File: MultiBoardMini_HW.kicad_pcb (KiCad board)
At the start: 2 copper layers, 63 x 63 mm, 52 parts, among them J1 PB0, J2 PA10, J3 Conn_01x02_Male, J4 PA10, J6 Conn_01x04, SW1 PF1, SW2 RESET, SW3 SW_Push_DPDT, SW5 SW_Push_DPDT, T3 PTS_1.5_2, U1 M78AR5-1, U2 NUCLEO-F303K8, U3 ESP32-C3-WROOM-02-N4, U4 TB67H303HG, U5 TB67H303HG, U6 MCP2562-E_SN

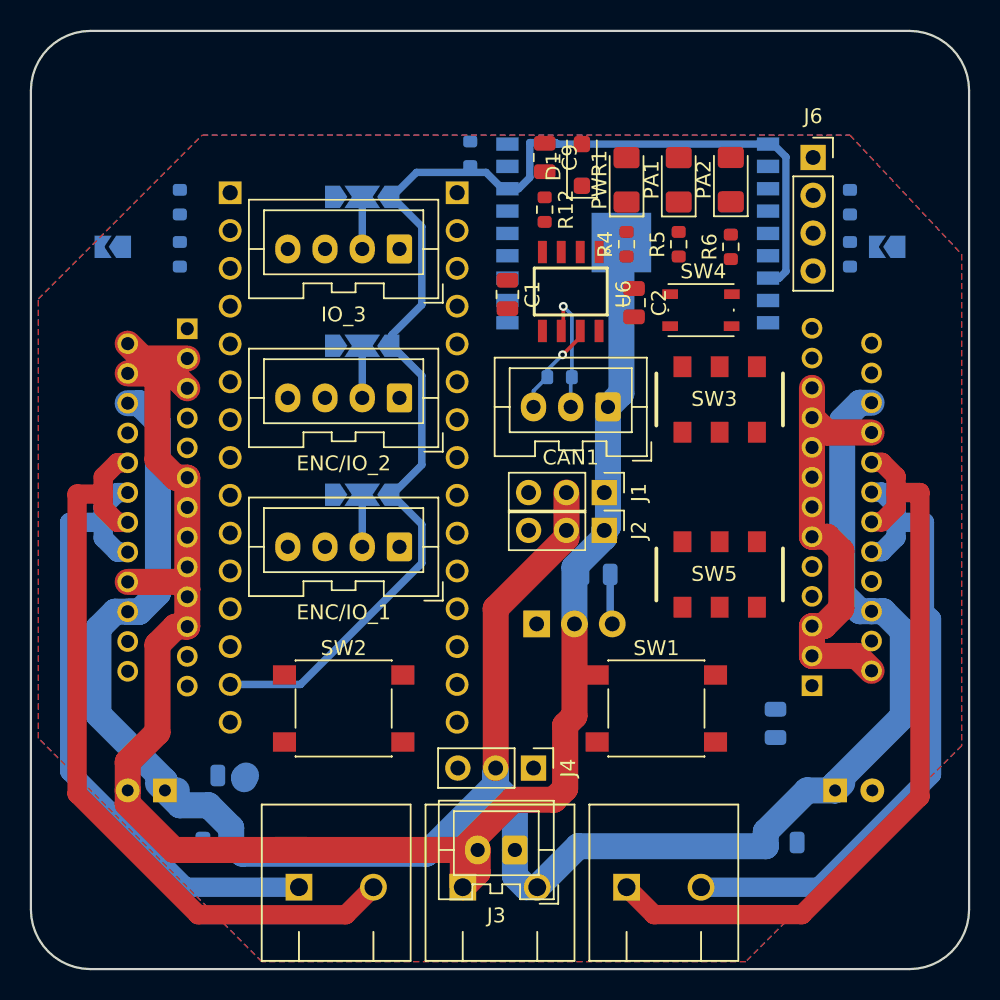
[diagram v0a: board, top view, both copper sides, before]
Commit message: 配線一応できた
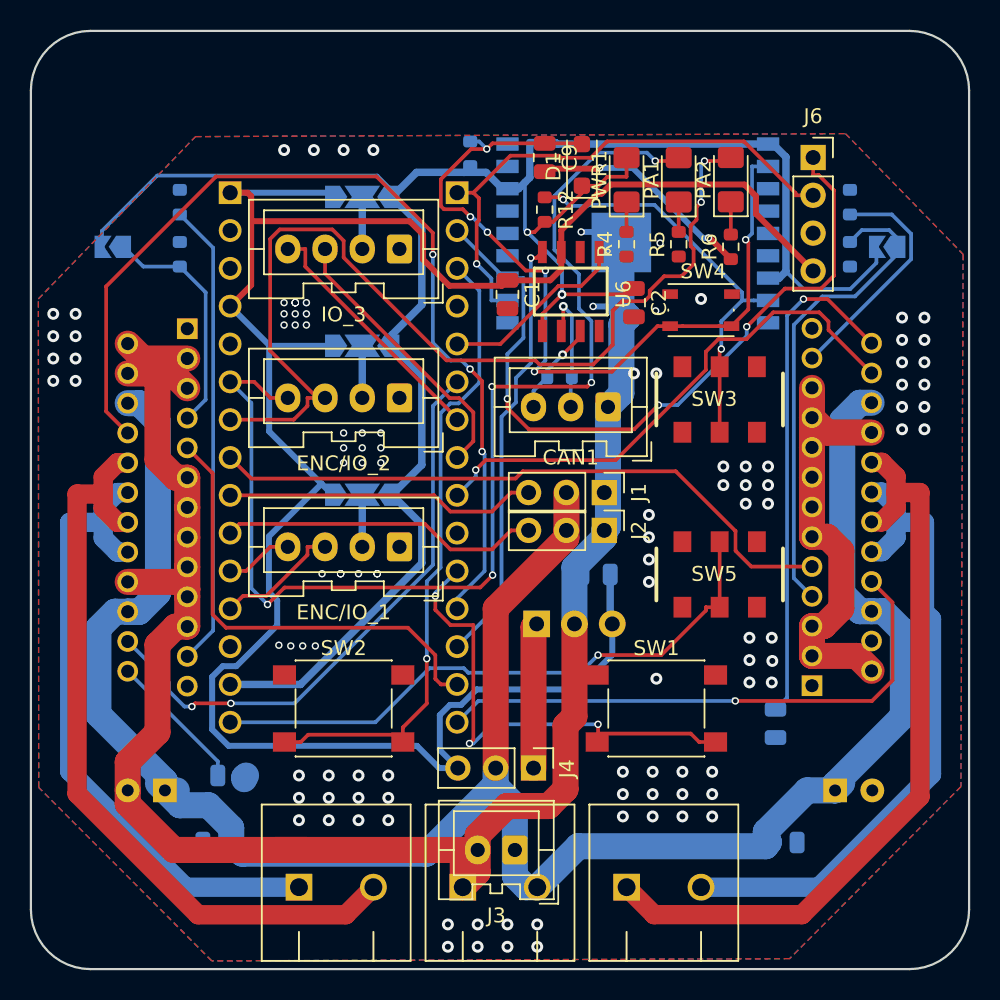
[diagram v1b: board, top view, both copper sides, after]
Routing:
- net +5V: track 3.38 -> 145.1 mm
- net Net-(ENC/IO_2-Pin_4): track 0.00 -> 79.1 mm, vias 0 -> 5
- net Net-(ENC/IO_2-Pin_3): track 0.00 -> 66.0 mm, vias 0 -> 2
- net Net-(U2A-PA8): track 0.00 -> 64.9 mm, vias 0 -> 3
- net +3V3: track 84.7 -> 142.9 mm, vias 0 -> 2
- net Net-(D1-A): track 0.00 -> 56.5 mm, vias 0 -> 6
- net Net-(J6-Pin_1): track 0.00 -> 50.8 mm, vias 0 -> 3
- net Net-(U2B-PA5): track 0.00 -> 43.3 mm
- net Net-(U2A-NRST_1): track 0.00 -> 43.0 mm, vias 0 -> 1
- net Net-(U2B-PB3): track 0.00 -> 40.9 mm, vias 0 -> 1
- net Net-(U2A-PB0): track 0.00 -> 39.5 mm, vias 0 -> 2
- net Net-(U2A-PB4): track 0.00 -> 37.8 mm, vias 0 -> 1
- net Net-(J6-Pin_2): track 0.00 -> 36.0 mm, vias 0 -> 1
- net Net-(U2A-PB1): track 0.00 -> 35.9 mm, vias 0 -> 1
- net Net-(U4-VREG): track 0.00 -> 34.1 mm, vias 0 -> 1
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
